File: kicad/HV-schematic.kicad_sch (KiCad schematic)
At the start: 13 parts, among them J0 Power in, J1 Power JST, J2 Steer motor JST, J3 Brake motor JST, J4 Steer motor out, J5 Hall sensor, J6 Brake motor out, U0 Relay, U1 ESCON_module-50/5, U2 A4988

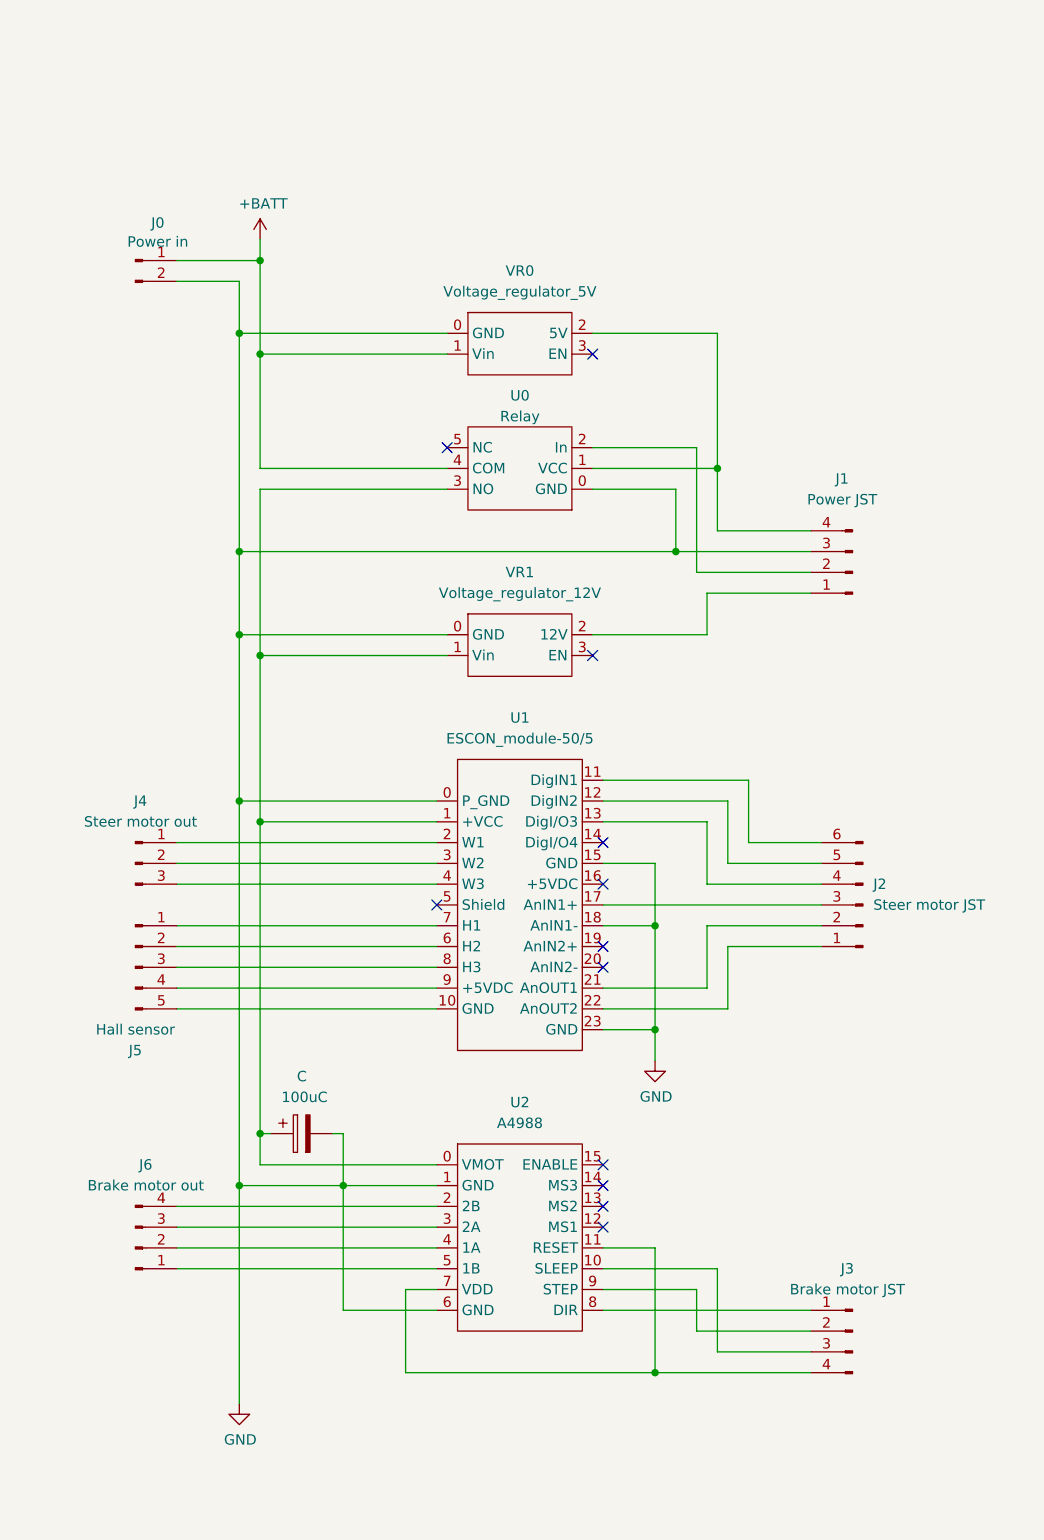
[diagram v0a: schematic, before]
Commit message: Update kicad and doc
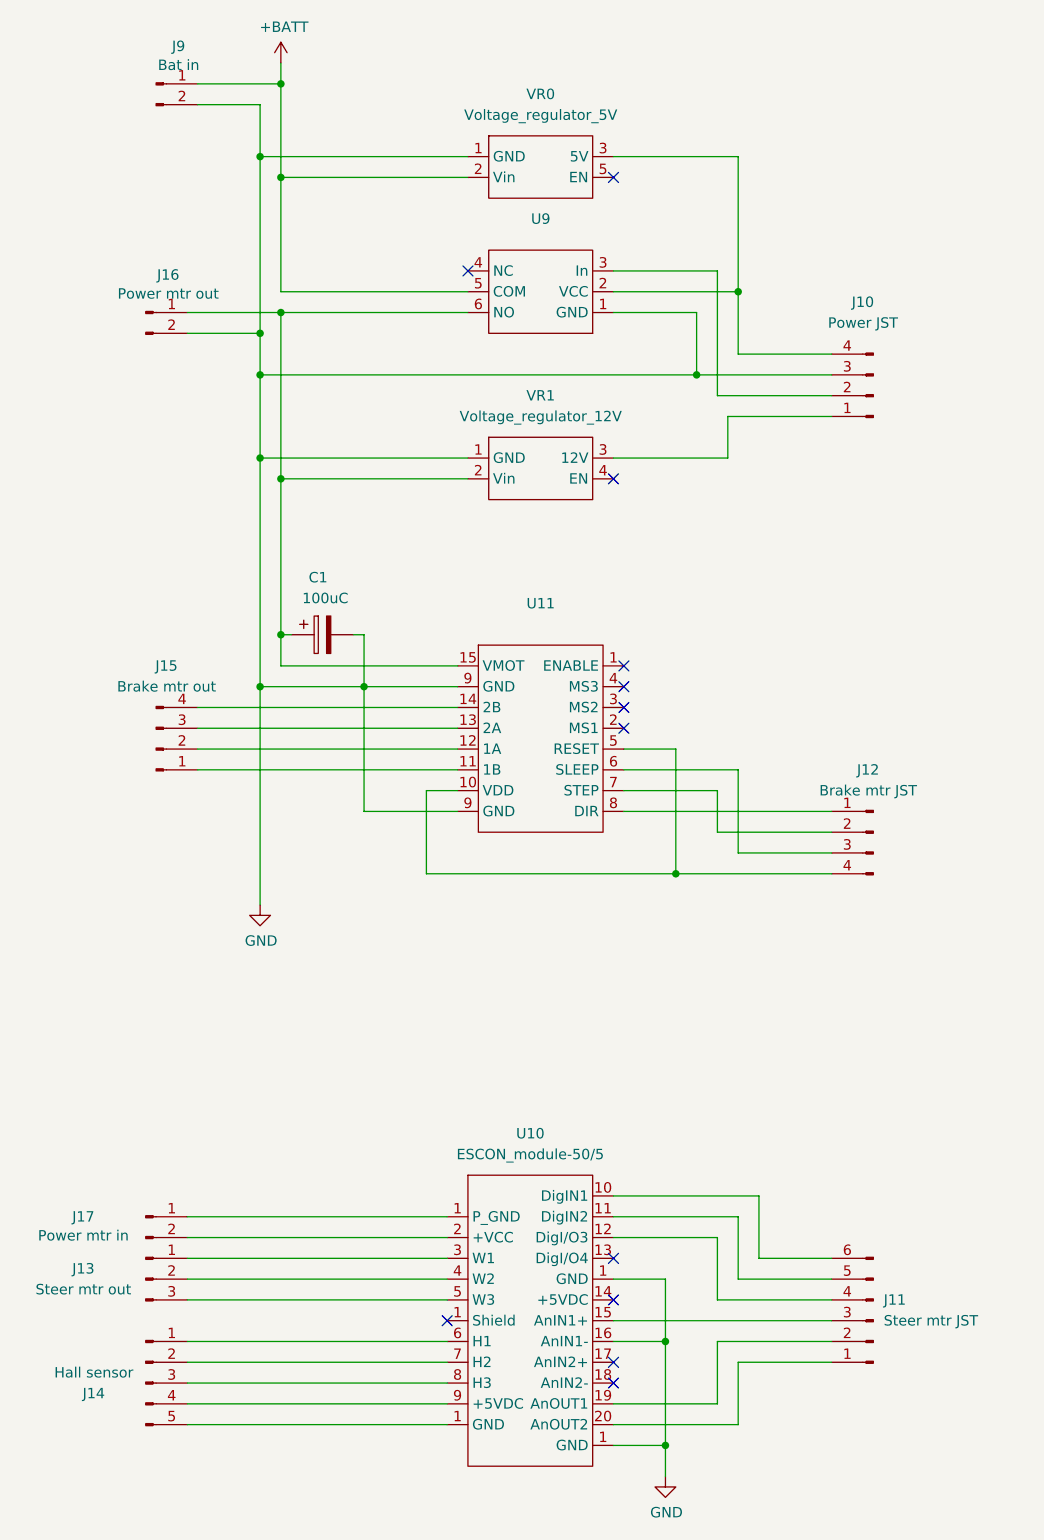
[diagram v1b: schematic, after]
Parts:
- added J16: Power mtr out, TerminalBlock:TerminalBlock_bornier-2_P5.08mm, symbol Connector:Conn_01x02_Male
- added J17: Power mtr in, symbol Connector:Conn_01x02_Male
- J10: renamed from J1; footprint (none) -> Connector_JST_inches:JST_1x04_P2.54
- J11: renamed from J2; value Steer motor JST -> Steer mtr JST
- J12: renamed from J3; value Brake motor JST -> Brake mtr JST; footprint (none) -> Connector_JST_inches:JST_1x04_P2.54
- J13: renamed from J4; value Steer motor out -> Steer mtr out
- J15: renamed from J6; value Brake motor out -> Brake mtr out; footprint (none) -> Connector_JST_inches:JST_1x04_P2.54
- J9: renamed from J0; value Power in -> Bat in
- U11: renamed from U2; value A4988 -> (none)
- U9: renamed from U0; value Relay -> (none)
- renumbered C to C1, J5 to J14, U1 to U10
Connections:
- net +BATT: now also U9.5 (COM), VR0.2 (Vin); no longer U9.4 (COM), VR0.1 (Vin)
- net GND: now also U10.1 (Shield), U10.16 (AnIN1-), U11.9 (GND), U9.1 (GND), VR0.1 (GND), VR1.1 (GND), J16.2 (Pin_2); no longer U10.0 (P_GND), U10.15 (GND), U10.18 (AnIN1-), U10.23 (GND), U11.1 (GND), U11.6 (GND), U9.0 (GND), VR0.0 (GND), VR1.0 (GND)
- net at U9.2 (VCC): now also J10.4 (Pin_4), VR0.3 (5V); no longer J10.2 (Pin_2)
- net at J15.1 (Pin_1): now also U11.11 (1B); no longer U11.5 (1B)
- net at J15.2 (Pin_2): now also U11.12 (1A); no longer U11.4 (1A)
- net at J15.3 (Pin_3): now also U11.13 (2A); no longer U11.3 (2A)
- net at J15.4 (Pin_4): now also U11.14 (2B); no longer U11.2 (2B)
- net at J14.5 (Pin_5): now also U10.1 (Shield); no longer U10.10 (GND)
- net at J11.6 (Pin_6): now also U10.10 (DigIN1); no longer U10.11 (DigIN1)
- net at J11.5 (Pin_5): now also U10.11 (DigIN2); no longer U10.12 (DigIN2)
- net at J11.4 (Pin_4): now also U10.12 (DigI/O3); no longer U10.13 (DigI/O3)
- net at J11.3 (Pin_3): now also U10.15 (AnIN1+); no longer U10.17 (AnIN1+)
- net at U10.19 (AnOUT1): now also J11.2 (Pin_2)
- net at U10.2 (+VCC): now also J17.2 (Pin_2); no longer J13.1 (Pin_1)
- net at U10.20 (AnOUT2): now also J11.1 (Pin_1)
- net at U10.3 (W1): now also J13.1 (Pin_1); no longer J13.2 (Pin_2)
- net at U10.4 (W2): now also J13.2 (Pin_2); no longer J13.3 (Pin_3)
- net at U10.5 (W3): now also J13.3 (Pin_3)
- net at U10.6 (H1): now also J14.1 (Pin_1); no longer J14.2 (Pin_2)
- net at U10.7 (H2): now also J14.2 (Pin_2); no longer J14.1 (Pin_1)
- net at U11.10 (VDD): now also J12.4 (Pin_4), U11.5 (RESET); no longer J12.3 (Pin_3)
- net at U11.15 (VMOT): now also C1.1, U9.6 (NO), VR1.2 (Vin), J16.1 (Pin_1)
- net at J12.2 (Pin_2): now also U11.7 (STEP); no longer U11.9 (STEP)
- net at J10.1 (Pin_1): now also VR1.3 (12V); no longer VR1.2 (12V)
- new net: J10.2 (Pin_2), U9.3 (In)
- new net: J17.1 (Pin_1), U10.1 (Shield)
- new net: J12.3 (Pin_3), U11.6 (SLEEP)
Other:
- moved on the sheet: C1, J10, J11, J12, J13, J14, J15, J9, U10, U11, U9, VR0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
